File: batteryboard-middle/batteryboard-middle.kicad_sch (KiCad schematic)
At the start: 8 parts, among them J1 FLE-105-01-G-DV-A, J2 Conn_01x02, J3 Conn_01x02, J4 FTS-105-01-L-DV-A

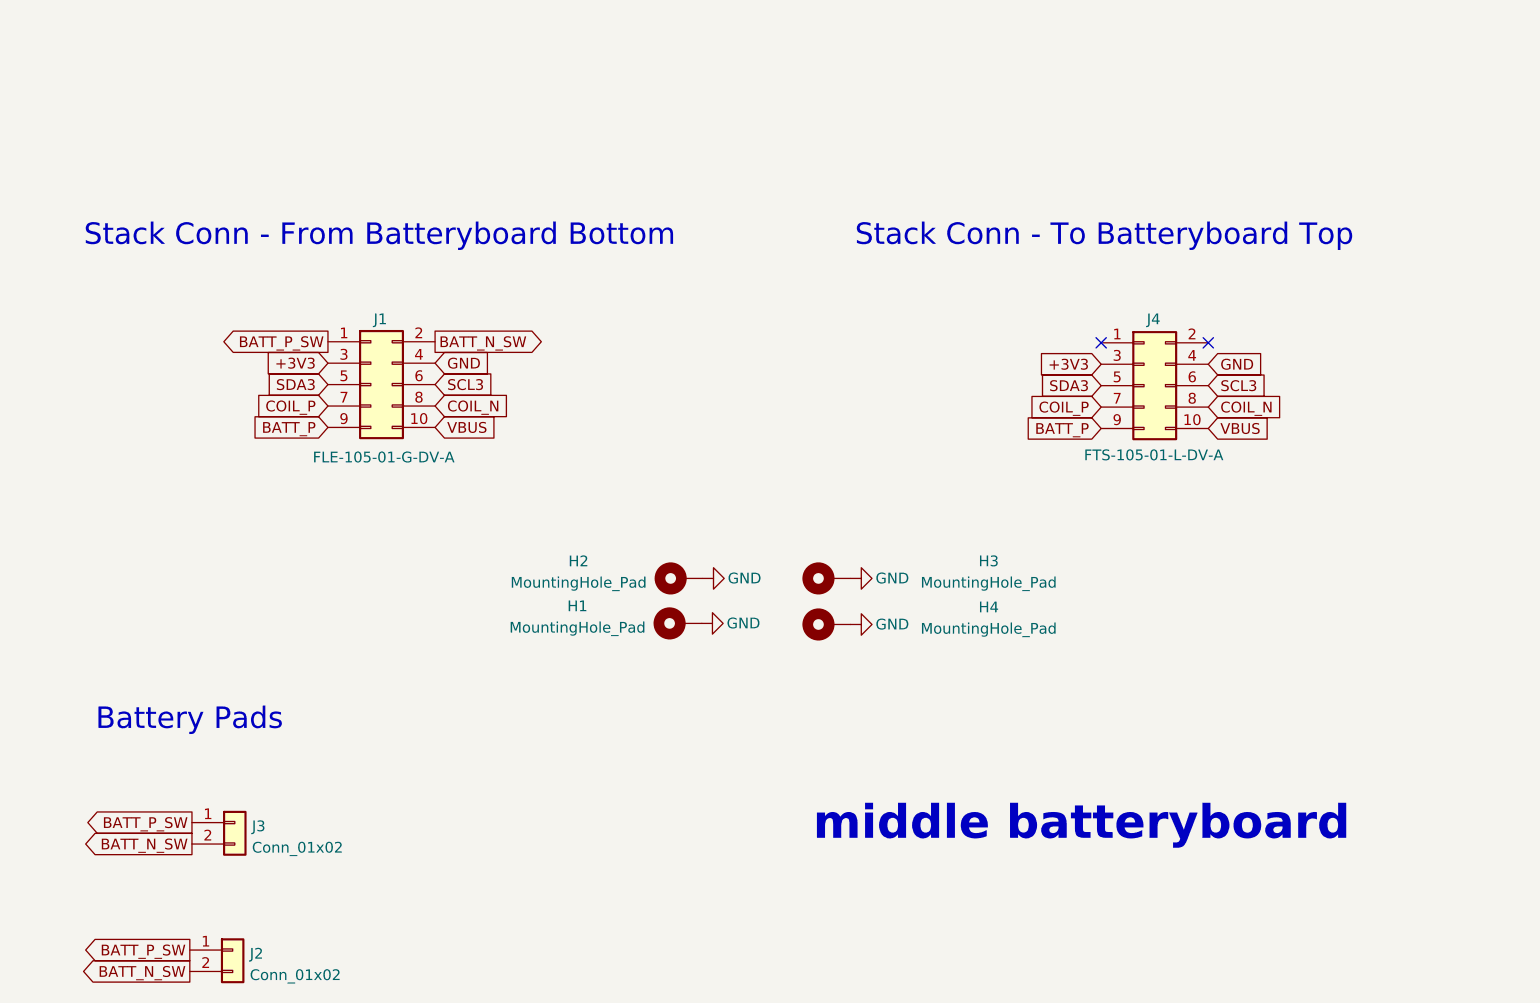
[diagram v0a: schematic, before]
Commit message: v02 Updates
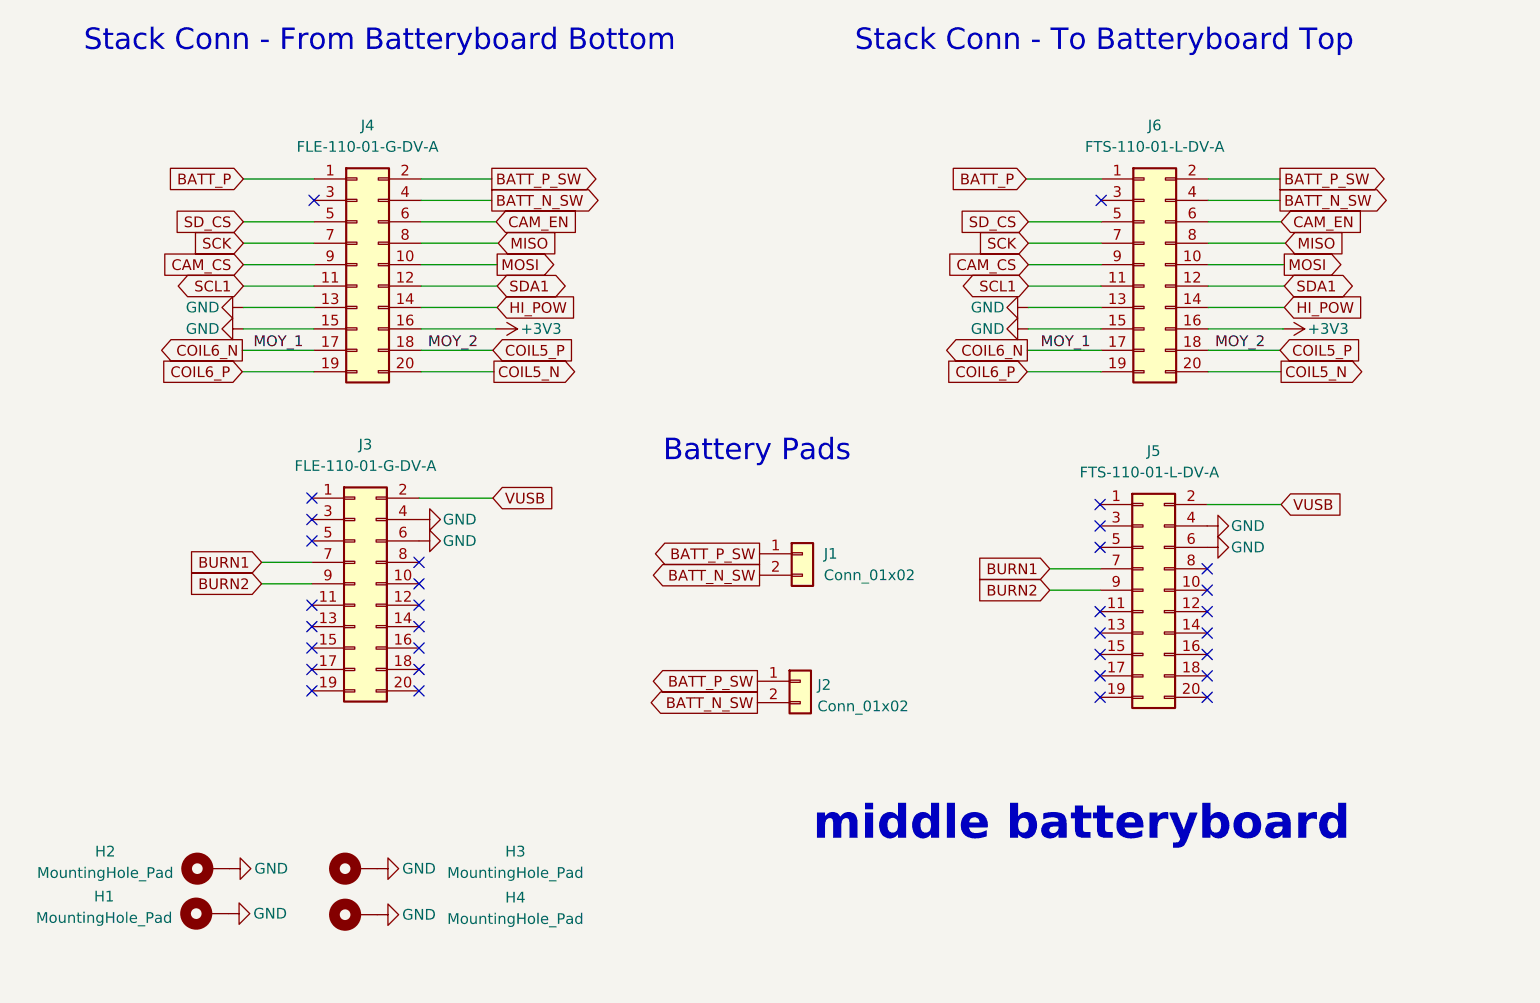
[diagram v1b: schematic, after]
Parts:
- removed J1: FLE-105-01-G-DV-A, batteryboard:SAMTEC_FLE-105-01-G-DV-A, symbol Connector_Generic:Conn_02x05_Odd_Even
- removed J4: FTS-105-01-L-DV-A, batteryboard:FTS-105-XX-YY-DV-A, symbol Connector_Generic:Conn_02x05_Odd_Even
- added J3, J4: FLE-110-01-G-DV-A, mainboard:SAMTEC_FLE-110-01-G-DV-A, symbol Connector_Generic:Conn_02x10_Odd_Even
- added J5, J6: FTS-110-01-L-DV-A, batteryboard:SAMTEC-FTS-110-01-X-DV-A, symbol Connector_Generic:Conn_02x10_Odd_Even
- renumbered J3 to J1
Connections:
- net +3V3: now also J4.16 (Pin_16), J6.16 (Pin_16)
- net BATT_N_SW: now also J4.4 (Pin_4), J6.4 (Pin_4)
- net BATT_P: now also J4.1 (Pin_1), J6.1 (Pin_1)
- net BATT_P_SW: now also J4.2 (Pin_2), J6.2 (Pin_2)
- net GND: now also J3.4 (Pin_4), J3.6 (Pin_6), J4.13 (Pin_13), J4.15 (Pin_15), J5.4 (Pin_4), J5.6 (Pin_6), J6.13 (Pin_13), J6.15 (Pin_15)
- new net BURN1: J3.7 (Pin_7), J5.7 (Pin_7)
- new net BURN2: J3.9 (Pin_9), J5.9 (Pin_9)
- new net CAM_CS: J4.9 (Pin_9), J6.9 (Pin_9)
- new net CAM_EN: J4.6 (Pin_6), J6.6 (Pin_6)
- new net COIL5_N: J4.20 (Pin_20), J6.20 (Pin_20)
- new net COIL5_P: J4.18 (Pin_18), J6.18 (Pin_18)
- new net COIL6_N: J4.17 (Pin_17), J6.17 (Pin_17)
- new net COIL6_P: J4.19 (Pin_19), J6.19 (Pin_19)
- new net HI_POW: J4.14 (Pin_14), J6.14 (Pin_14)
- new net MISO: J4.8 (Pin_8), J6.8 (Pin_8)
- new net MOSI: J4.10 (Pin_10), J6.10 (Pin_10)
- new net SCK: J4.7 (Pin_7), J6.7 (Pin_7)
- new net SCL1: J4.11 (Pin_11), J6.11 (Pin_11)
- new net SDA1: J4.12 (Pin_12), J6.12 (Pin_12)
- new net SD_CS: J4.5 (Pin_5), J6.5 (Pin_5)
- new net VUSB: J3.2 (Pin_2), J5.2 (Pin_2)
- no-connect marks 2 -> 32
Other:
- moved on the sheet: H1, H2, H3, H4, J1, J2
